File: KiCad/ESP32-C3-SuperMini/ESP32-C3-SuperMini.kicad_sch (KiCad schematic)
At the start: 39 parts, among them J1 USB_C_Receptacle_USB2.0_14P, SW1 SW_Push, SW2 SW_Push, U1 ESP32-C3, U2 ME6211C33M5G, Y1 Crystal_GND24

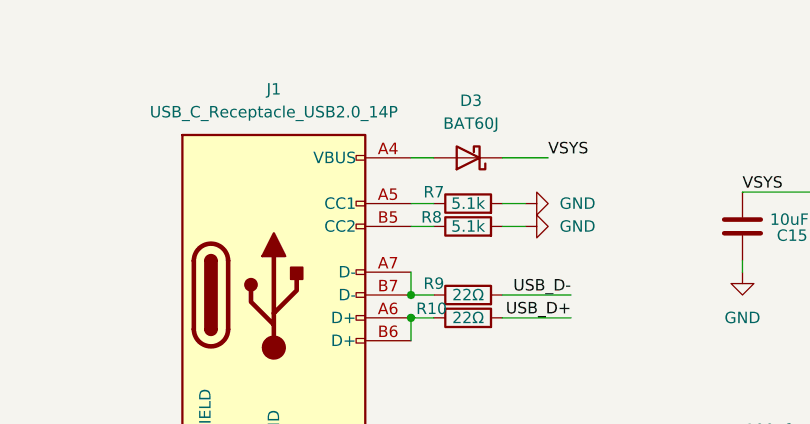
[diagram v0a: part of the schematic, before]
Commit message: wip
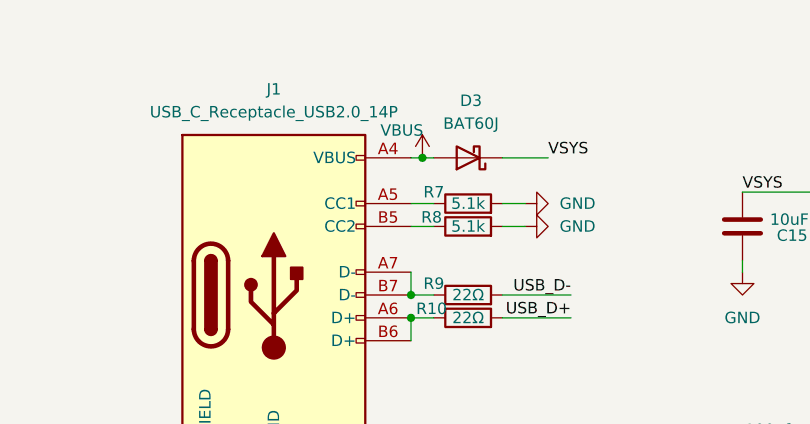
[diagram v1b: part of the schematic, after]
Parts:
- C5: footprint Capacitor_SMD:C_0201_0603Metric -> Capacitor_SMD:C_0402_1005Metric
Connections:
- net VBUS: now also D3.2 (A), J1.A4 (VBUS), J1.A9 (VBUS), J1.B4 (VBUS), J1.B9 (VBUS)
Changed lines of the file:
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@@
 	)
 	(junction
+		(at 68.58 29.21)
+		(diameter 0)
+		(color 0 0 0 0)
+	)
+	(junction
 		(at 106.68 60.96)
 		(diameter 0)
@@
 	(wire
 		(pts
-			(xy 67.31 29.21) (xy 69.85 29.21)
+			(xy 67.31 29.21) (xy 68.58 29.21)
 		)
 		(stroke
@@
 	(wire
 		(pts
+			(xy 68.58 29.21) (xy 69.85 29.21)
+		)
+		(stroke
+			(width 0)
+			(type default)
+		)
+	)
+	(wire
+		(pts
 			(xy 45.72 138.43) (xy 73.66 138.43)
 		)
@@
 	)
 	(symbol
+		(lib_id "power:VBUS")
+		(at 68.58 29.21 0)
+		(unit 1)
+		(exclude_from_sim no)
+		(in_bom yes)
+		(on_board yes)
+		(dnp no)
+		(property "Reference" "#PWR032"
+			(at 68.58 33.02 0)
+			(effects
+				(font
+					(size 1.27 1.27)
+				)
+				(hide yes)
+			)
+		)
+		(property "Value" "VBUS"
+			(at 66.294 26.162 0)
+			(effects
+				(font
+					(size 1.27 1.27)
+				)
+			)
+		)
+		(property "Footprint" ""
+			(at 68.58 29.21 0)
+			(effects
+				(font
+					(size 1.27 1.27)
+				)
+				(hide yes)
+			)
+		)
+		(property "Datasheet" ""
+			(at 68.58 29.21 0)
+			(effects
+				(font
+					(size 1.27 1.27)
+				)
+				(hide yes)
+			)
+		)
+		(property "Description" "Power symbol creates a global label with name \"VBUS\""
+			(at 68.58 29.21 0)
+			(effects
+				(font
+					(size 1.27 1.27)
+				)
+				(hide yes)
+			)
+		)
+		(pin "1"
+		)
+		(instances
+			(project "ESP32-C3-SuperMini"
+				(path "/3214b25f-d40d-4eea-81fa-4d993d5a2119"
+					(reference "#PWR032")
+					(unit 1)
+				)
+			)
+		)
+	)
+	(symbol
 		(lib_id "Device:C")
 		(at 110.49 76.2 0)
@@
 			)
 		)
-		(property "Footprint" "Capacitor_SMD:C_0201_0603Metric"
+		(property "Footprint" "Capacitor_SMD:C_0402_1005Metric"
 			(at 93.6752 95.25 0)
 			(effects

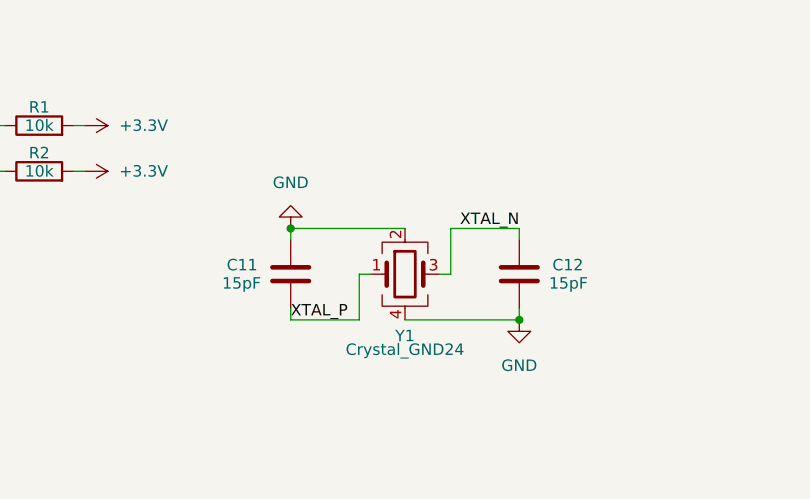
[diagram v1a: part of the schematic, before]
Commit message: v1?
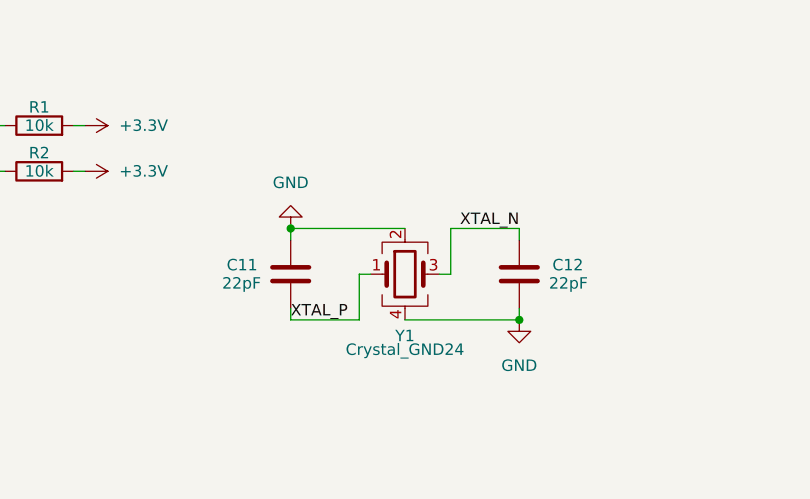
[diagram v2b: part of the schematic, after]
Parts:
- AE1: MPN 2450AT18A0100001E -> 2450AT18A0100001
- C11, C12: value 15pF -> 22pF
- Y1: LCSC (none) -> C9010; MPN (none) -> X322540MPB4SI
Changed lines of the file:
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@@
 			)
 		)
-		(property "MPN" "2450AT18A0100001E"
+		(property "MPN" "2450AT18A0100001"
 			(at 27.94 100.33 90)
 			(effects
@@
 			)
 		)
-		(property "Value" "15pF"
+		(property "Value" "22pF"
 			(at 167.64 143.256 0)
 			(effects
@@
 			)
 		)
+		(property "MPN" "X322540MPB4SI"
+			(at 187.96 142.24 0)
+			(effects
+				(font
+					(size 1.27 1.27)
+				)
+				(hide yes)
+			)
+		)
+		(property "LCSC" "C9010"
+			(at 187.96 142.24 0)
+			(effects
+				(font
+					(size 1.27 1.27)
+				)
+				(hide yes)
+			)
+		)
 		(pin "2"
 		)
@@
 			)
 		)
-		(property "Value" "15pF"
+		(property "Value" "22pF"
 			(at 208.28 143.256 0)
 			(effects
